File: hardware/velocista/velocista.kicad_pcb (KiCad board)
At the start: 2 copper layers, 120 x 106.2 mm, 19 parts, among them J1 XT30, J2 Cable_PAD, J3 Cable_PAD, J4 QTR8a, SW1 SW_Push, SW3 SW_SPDT, U1 TB6612FNG, U2 Mini360, U3 ESP32_DEVKITC

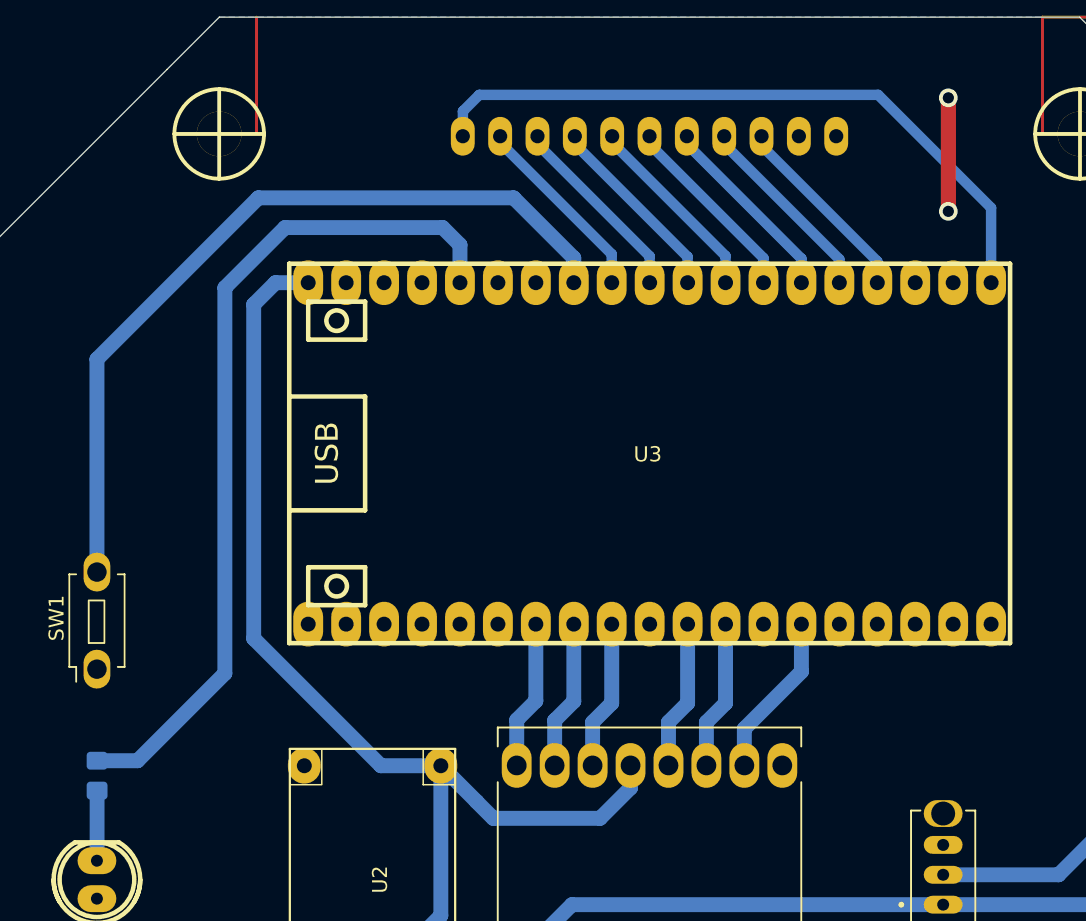
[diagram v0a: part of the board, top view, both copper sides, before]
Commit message: act placa
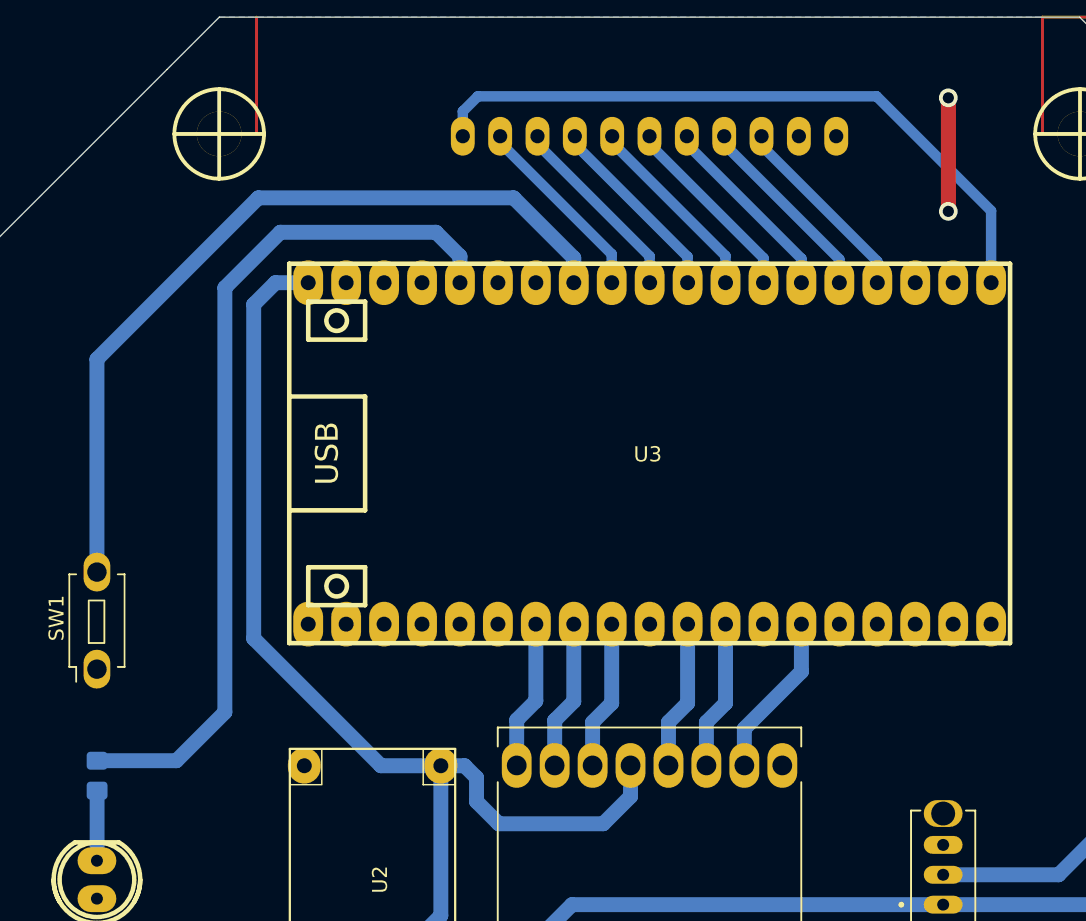
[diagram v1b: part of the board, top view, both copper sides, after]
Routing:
- net +5V: track 93.9 -> 95.4 mm
- net LED: track 57.2 -> 58.0 mm
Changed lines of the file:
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@@
 	)
 	(segment
-		(start 98.714366 87.006059)
-		(end 96.324366 84.616059)
+		(start 98.714366 87.014366)
+		(end 98.714366 85.414366)
 		(width 1)
 		(layer "B.Cu")
@@
 	)
 	(segment
-		(start 98.714366 87.016059)
-		(end 98.714366 87.006059)
-		(width 1)
-		(layer "B.Cu")
-		(net 1)
-	)
-	(segment
 		(start 103.944366 99.246059)
 		(end 103.944366 99.836059)
@@
 	)
 	(segment
+		(start 98.714366 85.414366)
+		(end 97.916059 84.616059)
+		(width 1)
+		(layer "B.Cu")
+		(net 1)
+	)
+	(segment
 		(start 83.794366 53.736059)
 		(end 85.254366 52.276059)
@@
 	)
 	(segment
-		(start 99.834366 88.136059)
-		(end 98.714366 87.016059)
-		(width 1)
-		(layer "B.Cu")
-		(net 1)
-	)
-	(segment
 		(start 85.254366 52.276059)
 		(end 87.444366 52.276059)
@@
 	)
 	(segment
-		(start 109.024366 86.096059)
-		(end 106.984366 88.136059)
+		(start 97.916059 84.616059)
+		(end 96.324366 84.616059)
 		(width 1)
 		(layer "B.Cu")
@@
 	)
 	(segment
+		(start 109.024366 86.675634)
+		(end 107.2 88.5)
+		(width 1)
+		(layer "B.Cu")
+		(net 1)
+	)
+	(segment
 		(start 103.944366 99.836059)
 		(end 103.944366 99.106059)
@@
 	)
 	(segment
-		(start 106.984366 88.136059)
-		(end 99.834366 88.136059)
+		(start 107.2 88.5)
+		(end 100.2 88.5)
 		(width 1)
 		(layer "B.Cu")
@@
 	)
 	(segment
+		(start 100.2 88.5)
+		(end 98.714366 87.014366)
+		(width 1)
+		(layer "B.Cu")
+		(net 1)
+	)
+	(segment
 		(start 83.794366 76.096059)
 		(end 83.794366 53.736059)
@@
 	)
 	(segment
-		(start 109.024366 84.596059)
-		(end 109.024366 86.096059)
-		(width 1)
-		(layer "B.Cu")
-		(net 1)
-	)
-	(segment
 		(start 103.944366 99.836059)
 		(end 103.944366 102.846059)
+		(width 1)
+		(layer "B.Cu")
+		(net 1)
+	)
+	(segment
+		(start 109.024366 84.596059)
+		(end 109.024366 86.675634)
 		(width 1)
 		(layer "B.Cu")
@@
 	)
 	(segment
-		(start 97.8 42.465425)
-		(end 97.8 40.8)
+		(start 133.164366 47.464366)
+		(end 133.164366 52.276059)
 		(width 0.7)
 		(layer "B.Cu")
@@
 	)
 	(segment
-		(start 97.8 40.8)
-		(end 98.9 39.7)
+		(start 98.8 39.8)
+		(end 125.5 39.8)
 		(width 0.7)
 		(layer "B.Cu")
@@
 	)
 	(segment
-		(start 125.6 39.7)
-		(end 133.164366 47.264366)
-		(width 0.7)
-		(layer "B.Cu")
-		(net 10)
-	)
-	(segment
-		(start 98.9 39.7)
-		(end 125.6 39.7)
-		(width 0.7)
-		(layer "B.Cu")
-		(net 10)
-	)
-	(segment
-		(start 133.164366 47.264366)
-		(end 133.164366 52.276059)
-		(width 0.7)
-		(layer "B.Cu")
-		(net 10)
-	)
-	(segment
-		(start 81.864366 78.435634)
-		(end 76.02 84.28)
-		(width 1)
-		(layer "B.Cu")
-		(net 11)
-	)
-	(segment
-		(start 76.02 84.28)
+		(start 97.794366 40.805634)
+		(end 98.8 39.8)
+		(width 0.7)
+		(layer "B.Cu")
+		(net 10)
+	)
+	(segment
+		(start 125.5 39.8)
+		(end 133.164366 47.464366)
+		(width 0.7)
+		(layer "B.Cu")
+		(net 10)
+	)
+	(segment
+		(start 97.794366 42.471059)
+		(end 97.794366 40.805634)
+		(width 0.7)
+		(layer "B.Cu")
+		(net 10)
+	)
+	(segment
+		(start 81.864366 52.616059)
+		(end 81.864366 81.035634)
+		(width 1)
+		(layer "B.Cu")
+		(net 11)
+	)
+	(segment
+		(start 97.604366 52.276059)
+		(end 97.604366 50.504366)
+		(width 1)
+		(layer "B.Cu")
+		(net 11)
+	)
+	(segment
+		(start 81.864366 81.035634)
+		(end 78.62 84.28)
+		(width 1)
+		(layer "B.Cu")
+		(net 11)
+	)
+	(segment
+		(start 78.62 84.28)
 		(end 73.31 84.28)
 		(width 1)
@@
 	)
 	(segment
-		(start 97.604366 52.276059)
-		(end 97.604366 49.746059)
-		(width 1)
-		(layer "B.Cu")
-		(net 11)
-	)
-	(segment
-		(start 81.864366 52.616059)
-		(end 81.864366 78.435634)
-		(width 1)
-		(layer "B.Cu")
-		(net 11)
-	)
-	(segment
-		(start 96.444366 48.586059)
-		(end 85.894366 48.586059)
-		(width 1)
-		(layer "B.Cu")
-		(net 11)
-	)
-	(segment
-		(start 97.604366 49.746059)
-		(end 96.444366 48.586059)
-		(width 1)
-		(layer "B.Cu")
-		(net 11)
-	)
-	(segment
-		(start 85.894366 48.586059)
+		(start 97.604366 50.504366)
+		(end 96 48.9)
+		(width 1)
+		(layer "B.Cu")
+		(net 11)
+	)
+	(segment
+		(start 96 48.9)
+		(end 85.580425 48.9)
+		(width 1)
+		(layer "B.Cu")
+		(net 11)
+	)
+	(segment
+		(start 85.580425 48.9)
 		(end 81.864366 52.616059)
 		(width 1)
